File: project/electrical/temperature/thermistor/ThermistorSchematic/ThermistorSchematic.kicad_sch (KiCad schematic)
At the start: 12 parts, among them U1 MCP601, U2 MCP601

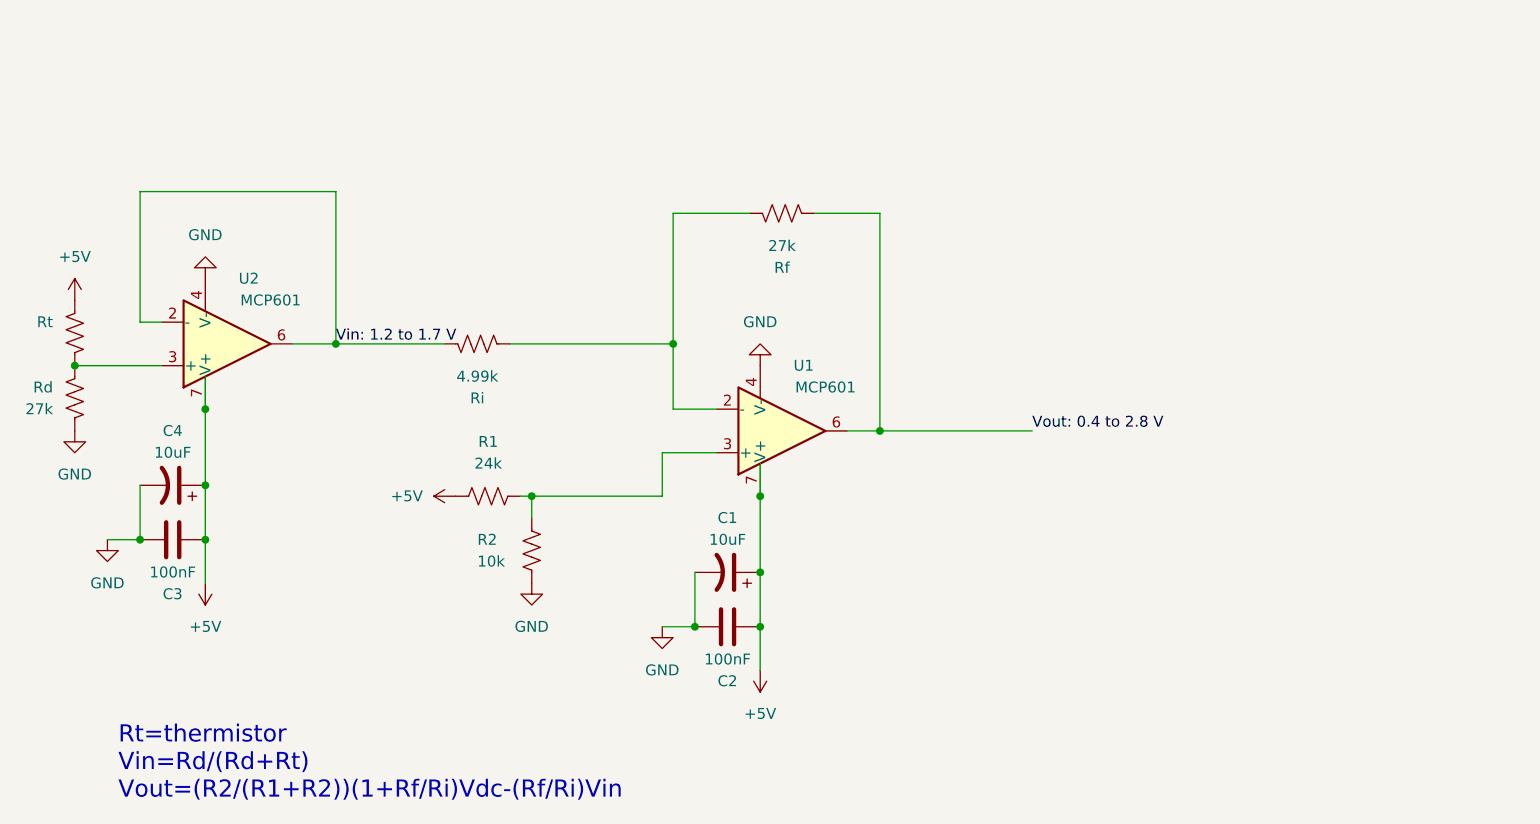
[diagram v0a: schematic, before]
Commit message: Made some circuits better for overleaf
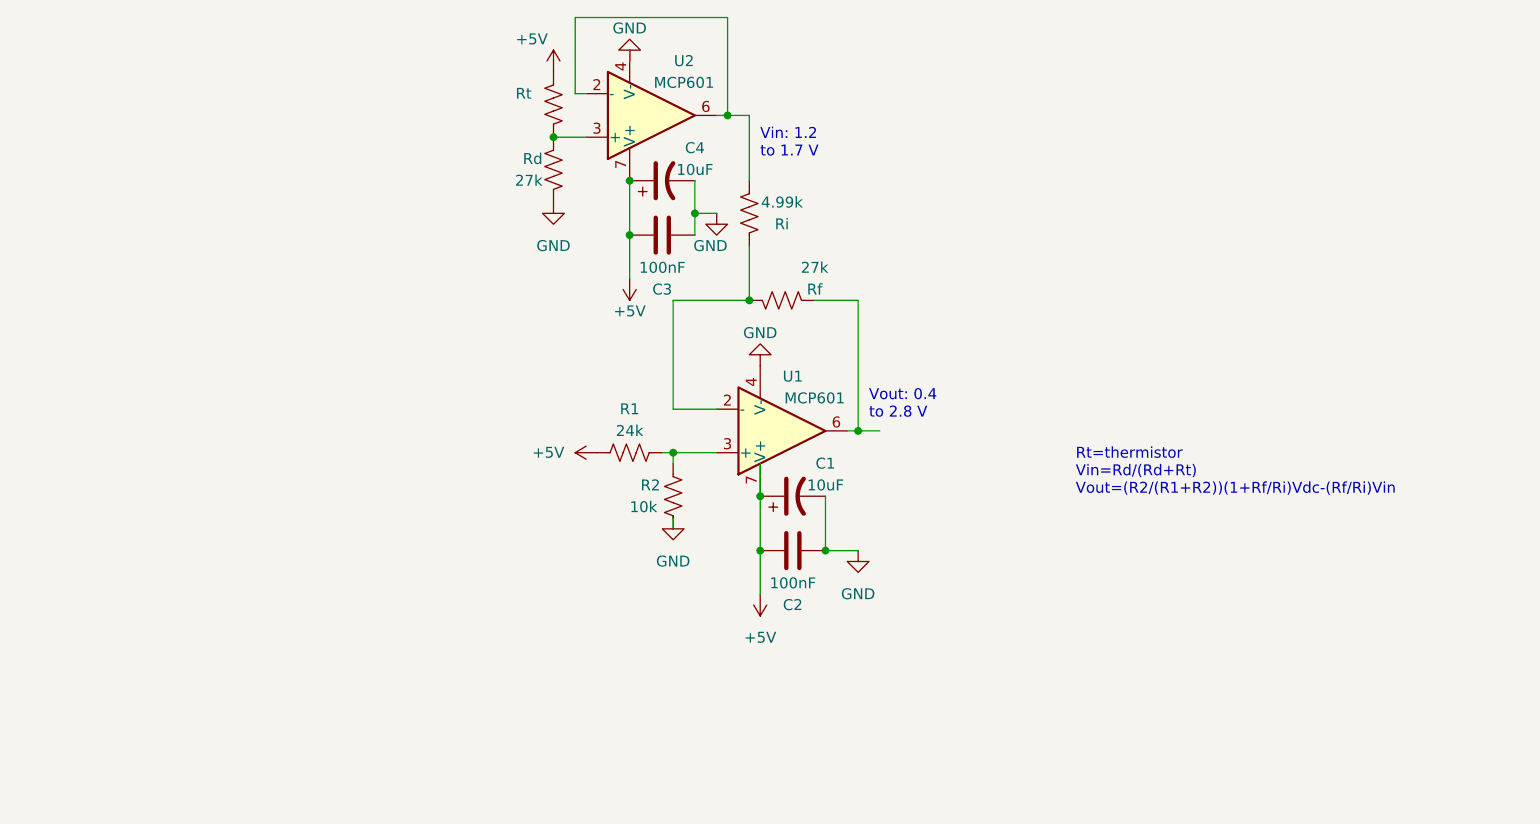
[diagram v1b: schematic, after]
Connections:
- net Vin: 1.2 to 1.7 V: no longer names the net of Ri.1, U2.2 (-), U2.6
- net Vout: 0.4 to 2.8 V: no longer names the net of Rf.2, U1.6
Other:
- note added: "Vin: 1.2 to 1.7 V"
- note added: "Vout: 0.4 to 2.8 V"
- moved on the sheet: C1, C2, C3, C4, R1, R2, Rd, Rf, Ri, Rt, U2
